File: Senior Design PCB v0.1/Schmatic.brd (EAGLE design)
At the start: 101.3 x 66.8 mm, 233 parts, among them IC1 TMC2208, IC2 TMC2208, IC3 TMC2208, IC4 TMC2208, IC5 TMC2208, IC6 CP2104, Q1 mmbt2222, Q2 mmbt2222, Q3 MMBT4403, Q4 AOD417, Q5 MMBT4403, Q6 MMBT4403, Q7 DMG3415U, U1 PCA9685, U2 AP2112-3.3, U3 HTU21DF, U4 HX711, U5 HX711, U6 HX711, U7 SX1509, X2 ESP32_WROOM32_SKINNY

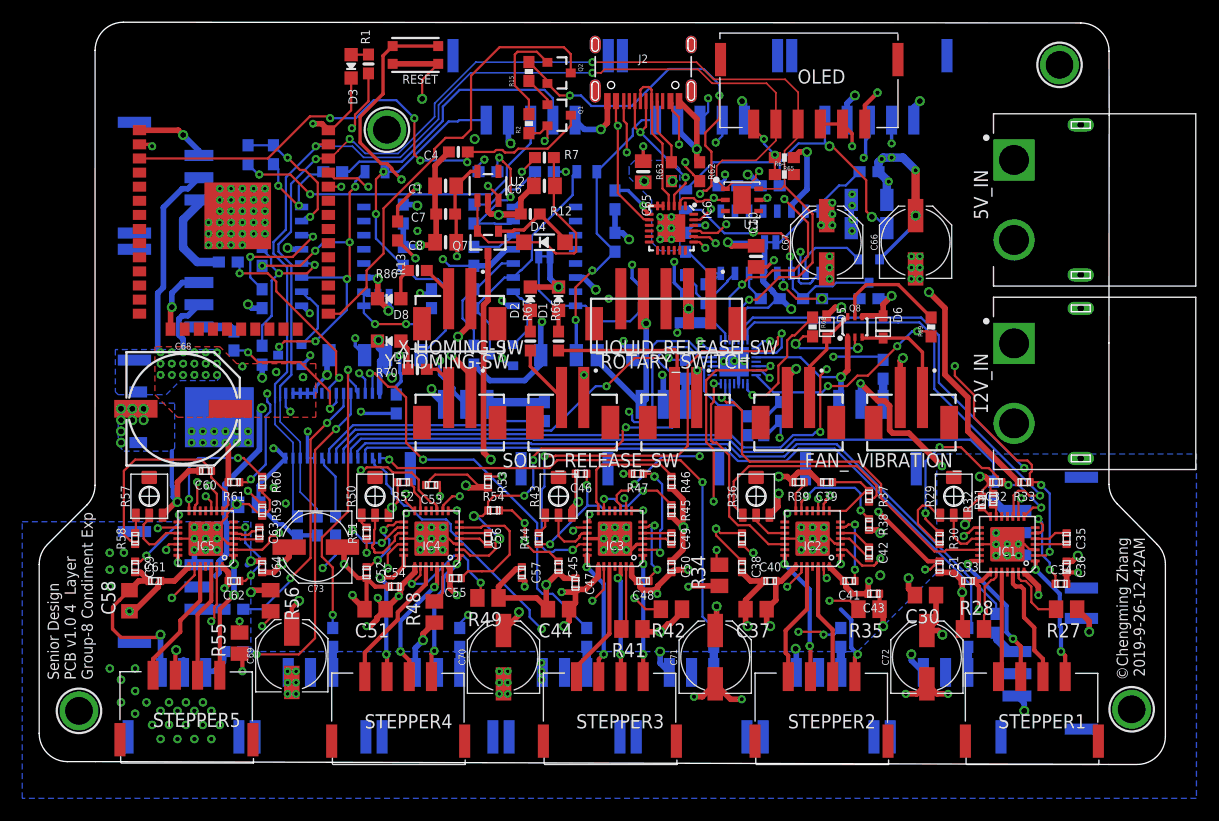
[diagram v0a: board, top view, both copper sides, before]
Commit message: added contact board
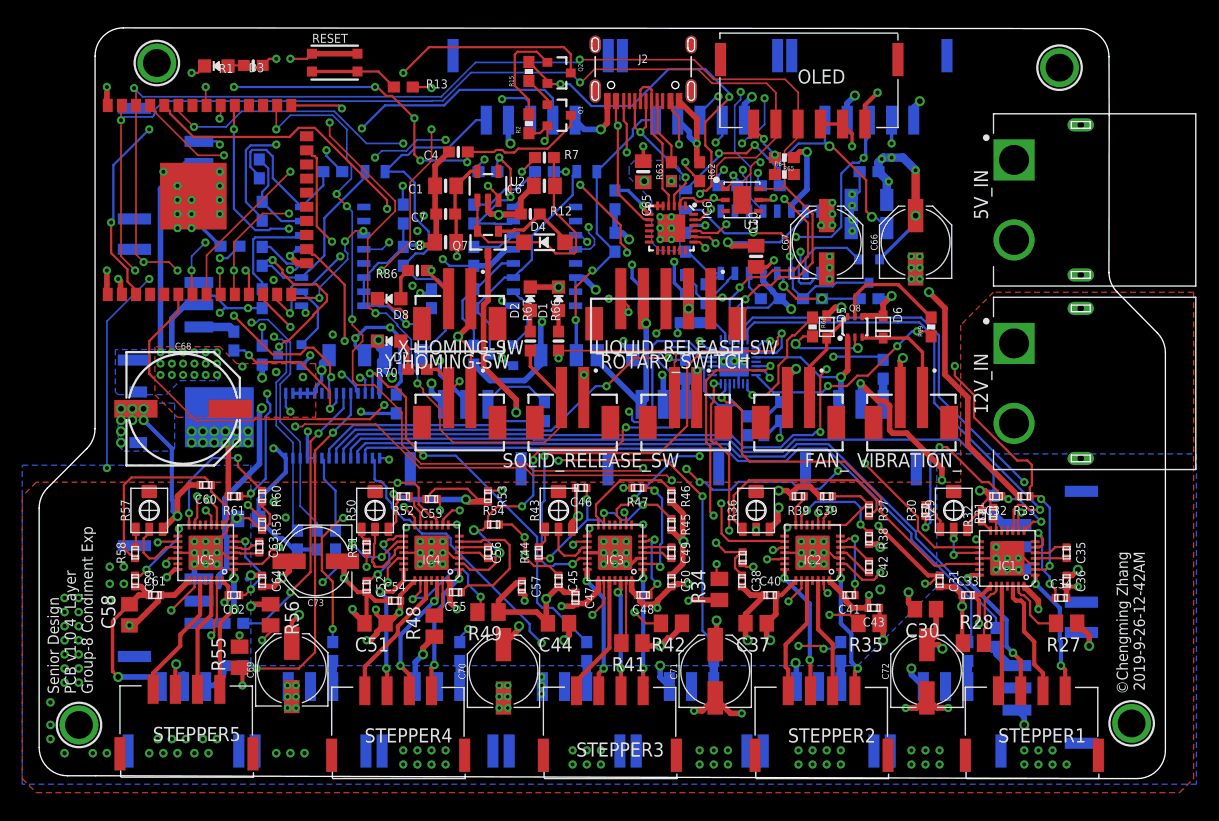
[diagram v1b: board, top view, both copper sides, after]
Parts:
- removed SJ1, SJ2, SJ3: JUMPER-PAD-2-NC_BY_TRACE, SparkFun-Passives:PAD-JUMPER-2-NC_BY_TRACE_YES_SILK
- moved U$49 21.6 mm to (4.50, 63.1)
- moved R13 13.0 mm to (26.7, 61.0), turned to 0 degrees
- moved D3 12.1 mm to (9.85, 62.8), turned to 90 degrees
- moved R1 10.4 mm to (13.2, 62.9), turned to 180 degrees
- moved RESET 7.30 mm to (20.5, 63.2), turned to 0 degrees
- moved X2 6.48 mm to (5.08, 50.8), turned to 90 degrees
- moved R22 5.24 mm to (14.0, 49.8)
- moved R30 2.84 mm to (73.7, 22.9), turned to 0 degrees
- moved C25 1.80 mm to (13.7, 53.6)
- moved R40 1.72 mm to (57.2, 18.6)
- moved R82 1.44 mm to (11.1, 46.6)
- moved R71 1.27 mm to (79.8, 23.3)
- moved SERVO12 1.27 mm to (90.2, 25.4)
- moved C33 1.27 mm to (77.5, 15.2)
- moved C37 1.27 mm to (58.4, 12.7)
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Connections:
- removed net A13_I35: X2.7
- removed net A2_I34: X2.6
- removed net A5_IO4: X2.26
- removed net BUZZER: X2.10
- removed net CAP_OR_BAT: X2.14
- removed net CHARGE_OR_NOT: X2.16
- removed net IO15_A8: X2.23
- removed net IO21: X2.33
- removed net IO32_A7: X2.8
- removed net MISO: X2.31
- removed net MOSI: X2.30
- removed net N$10: R16.1, SJ2.2, U4.15, U4.16
- removed net N$18: R21.1, SJ1.2, U5.15, U5.16
- removed net N$25: R26.1, SJ3.2, U6.15, U6.16
- removed net ONBOARD_LED: X2.13
- removed net RX_CUS: X2.12
- removed net SCK: X2.29
- removed net SD_CS_MCU: X2.9
- removed net TX_CUS: X2.11
- net GND: now also R16.1, R21.1, R26.1, U4.15, U4.16, U5.15, U5.16, U6.15, U6.16; no longer SJ1.1, SJ2.1, SJ3.1
- net LRSW: now also X2.16
- net ROTA_A: now also X2.33
- net ROTA_C: now also X2.12
- net ROTA_E: now also X2.23
- net SRSW: now also X2.30
- net STEP_1: now also X2.26
- net STEP_2: now also X2.29
- net STEP_LIQUID: now also X2.31
- net WEIGHT_CLK_1: now also X2.9
- net WEIGHT_CLK_2: now also X2.11
- net WEIGHT_CLK_3: now also X2.14
- net WEIGHT_DATA_1: now also X2.8
- net WEIGHT_DATA_2: now also X2.10
- net WEIGHT_DATA_3: now also X2.13
- net X-HOMING: now also X2.6
- net Y-HOMING: now also X2.7
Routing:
- net STEP_1: track 0.00 -> 102.0 mm, vias 0 -> 9
- net STEP_2: track 0.00 -> 83.7 mm, vias 0 -> 5
- net WEIGHT_CLK_1: track 0.00 -> 77.2 mm, vias 0 -> 6
- net WEIGHT_DATA_1: track 0.00 -> 70.5 mm, vias 0 -> 4
- net SRSW: track 5.39 -> 65.7 mm, vias 0 -> 4
- net ROTA_A: track 0.00 -> 58.7 mm, vias 0 -> 3
- net STEP_LIQUID: track 49.3 -> 105.5 mm, vias 5 -> 8
- net ROTA_E: track 0.00 -> 55.3 mm, vias 0 -> 3
- net WEIGHT_DATA_2: track 0.00 -> 42.0 mm, vias 0 -> 4
- net ROTA_C: track 0.00 -> 41.6 mm, vias 0 -> 2
- net X-HOMING: track 3.90 -> 45.2 mm, vias 0 -> 2
- net WEIGHT_CLK_2: track 0.00 -> 36.5 mm, vias 0 -> 3
- net LRSW: track 14.9 -> 46.7 mm, vias 0 -> 2
- net SDA: track 123.8 -> 154.7 mm, vias 5 -> 7
- net Y-HOMING: track 4.37 -> 33.0 mm, vias 0 -> 3
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- added copper zone on layer 1, net 12V_REG
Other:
- board size 101.3 x 66.8 mm -> 101.3 x 67.6 mm
